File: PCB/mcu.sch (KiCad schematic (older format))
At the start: 50 parts, among them J1 DBG, P1 PC, P2 Link, P3 SSD1107, Q1 SSP6206, U1 USBLC6-2SC6, U2 USBLC6-2SC6, U3 STM32F103CBTx

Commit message: Update YAEMK
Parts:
- removed C39: 100n, prettylib:SMD-0603, symbol YAEMK:C
- removed D78: LED, prettylib:LED-0603, symbol YAEMK:LED
- added C3, C38: 100n, prettylib:SMD-0603, symbol YAEMK:C
- added D38, D39: DIODE, Diode_SMD:D_0603_1608Metric, symbol YAEMK:DIODE
- added Q2: Q_PNP_BCE, prettylib:SOT-23, symbol Device:Q_PNP_BCE
- added R14: 1k5, prettylib:SMD-0603, symbol YAEMK:R
- added R15, R16: 33, prettylib:SMD-0603, symbol YAEMK:R
- added R8: 120R, prettylib:SMD-0603, symbol YAEMK:R
- added S7: DFU, prettylib:SMD_Tacticle_Switch_TS24CA, symbol YAEMK:SW
- added U4: 24LC64, Package_SO:TSSOP-8_4.4x3mm_P0.65mm, symbol Memory_EEPROM:24LC64
- JP10, JP3, JP4, JP5, JP6, JP7, JP8, JP9: symbol YAEMK:SolderJumper_2_Open -> YAEMK-rescue:SolderJumper_2_Open-YAEMK
- Q1: symbol YAEMK:SSP6206 -> YAEMK-rescue:SSP6206-YAEMK
- R10: value 10k -> 1M
- R9: value 2k2 -> 1k5
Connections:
- net labels added: BOOT0_CHARGE
- net labels removed: MCU_LED
- wire segments 150 -> 181
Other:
- note added: "I2C EEPROM"
- note added: "Reset and DFU Bootloader Circuit"
- note removed: "Boot Mode"
- note removed: "Reset Button\n"
- moved on the sheet: C37, C42, C43, C44, C45, C46, C47, C48, C49, C56, C57, C59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

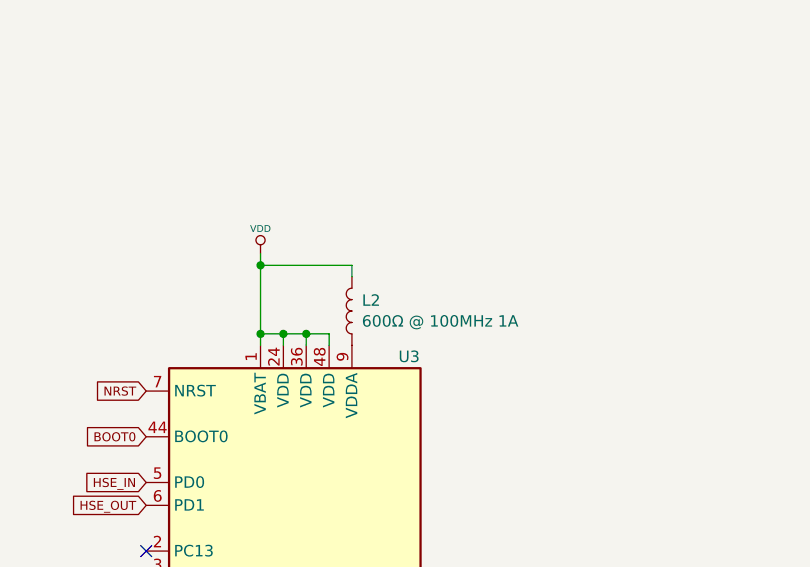
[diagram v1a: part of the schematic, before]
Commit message: Update YAEMK 1
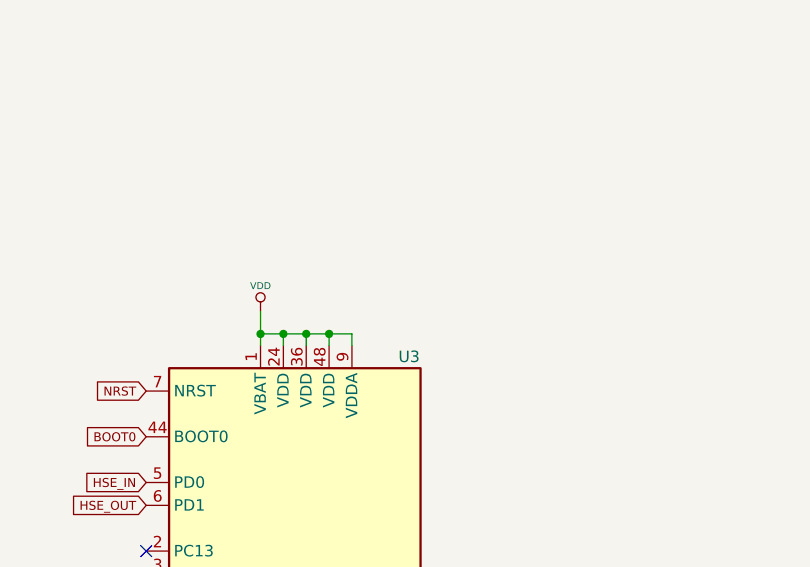
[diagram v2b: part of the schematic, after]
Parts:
- removed L2: 600Ω @ 100MHz 1A, prettylib:SMD-0603, symbol YAEMK:L
- HSE1: footprint prettylib:Crystal_SMD_EuroQuartz_MJ-4Pin_5.0x3.2mm -> Crystal:Crystal_SMD_3225-4Pin_3.2x2.5mm
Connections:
- net VDD: now also U3.9 (VDDA)
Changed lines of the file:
@@
 L YAEMK:VDD #PWR025
 U 1 1 5EA004DE
-P 8550 4450
-F 0 "#PWR025" H 8550 4550 30  0001 C CNN
-F 1 "VDD" H 8550 4560 30  0000 C CNN
-F 2 "" H 8550 4450 60  0000 C CNN
-F 3 "" H 8550 4450 60  0000 C CNN
-	1    8550 4450
+P 8550 4700
+F 0 "#PWR025" H 8550 4800 30  0001 C CNN
+F 1 "VDD" H 8550 4810 30  0000 C CNN
+F 2 "" H 8550 4700 60  0000 C CNN
+F 3 "" H 8550 4700 60  0000 C CNN
+	1    8550 4700
 	1    0    0    -1
 $EndComp
@@
 Wire Wire Line
 	8750 4800 8850 4800
-Wire Wire Line
-	8550 4450 8550 4500
 Wire Wire Line
 	8550 8000 8550 7900
@@
 F 0 "HSE1" H 14050 1300 50  0000 L CNN
 F 1 "8MHz" H 14050 1200 50  0000 L CNN
-F 2 "prettylib:Crystal_SMD_EuroQuartz_MJ-4Pin_5.0x3.2mm" H 14400 1050 50  0001 C CNN
+F 2 "Crystal:Crystal_SMD_3225-4Pin_3.2x2.5mm" H 14400 1050 50  0001 C CNN
 F 3 "~" H 14400 1050 50  0001 C CNN
 	1    14400 1050
@@
 	8650 4800 8750 4800
 $Comp
-L YAEMK:L L2
-U 1 1 5F849BB2
-P 8950 4700
-F 0 "L2" H 8907 4654 50  0000 R CNN
-F 1 "600Ω @ 100MHz 1A" H 8907 4745 50  0000 R CNN
-F 2 "prettylib:SMD-0603" H 8950 4700 50  0001 C CNN
-F 3 "~" H 8950 4700 50  0001 C CNN
-	1    8950 4700
-	-1   0    0    1
-$EndComp
-$Comp
 L YAEMK:VSS #PWR026
 U 1 1 5EAADE05
@@
 	1    0    0    -1
 $EndComp
-Wire Wire Line
-	8950 4550 8950 4500
-Wire Wire Line
-	8950 4500 8550 4500
-Connection ~ 8550 4500
-Wire Wire Line
-	8550 4500 8550 4800
 $Comp
 L YAEMK:USB_C_Receptacle_USB2.0 P1
@@
 Wire Wire Line
 	10350 7350 10150 7350
+Wire Wire Line
+	8550 4700 8550 4800
+Wire Wire Line
+	8950 4850 8950 4800
+Wire Wire Line
+	8950 4800 8850 4800
+Connection ~ 8850 4800
 $EndSCHEMATC

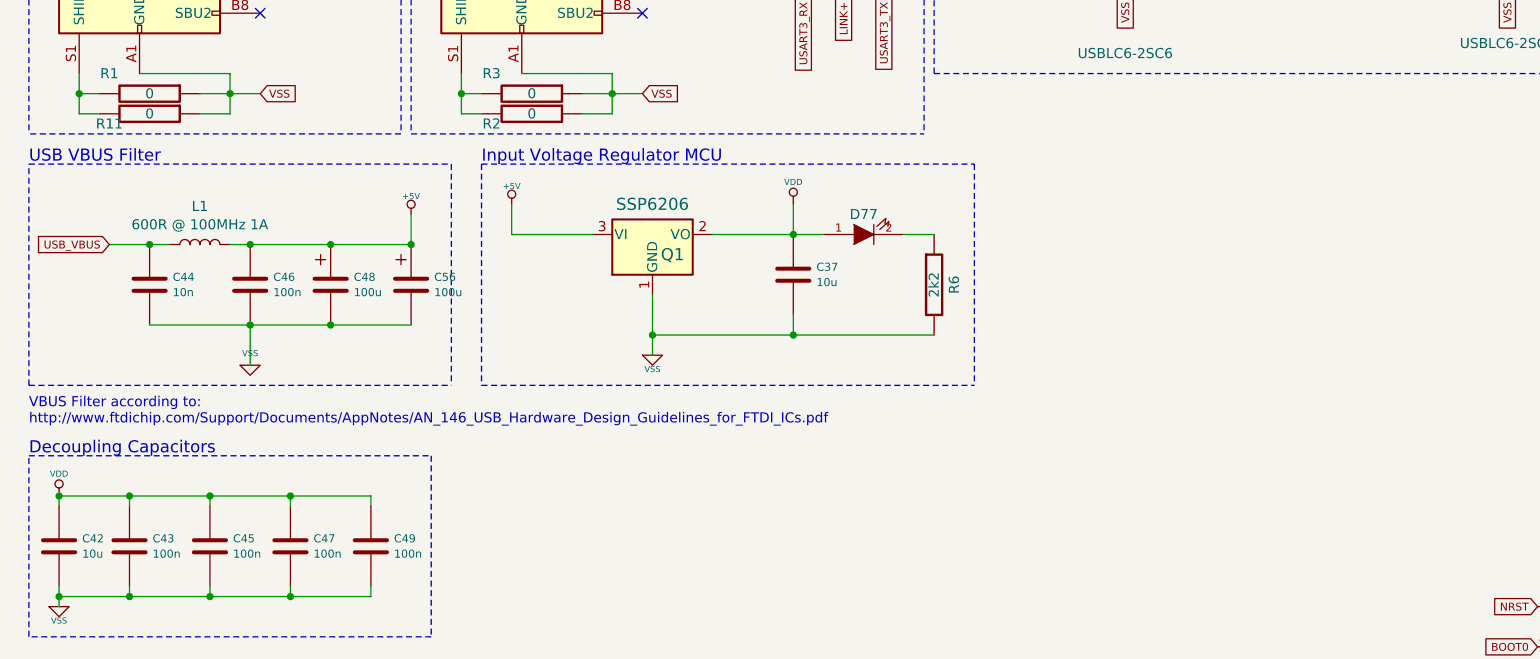
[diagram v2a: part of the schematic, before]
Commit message: Sync
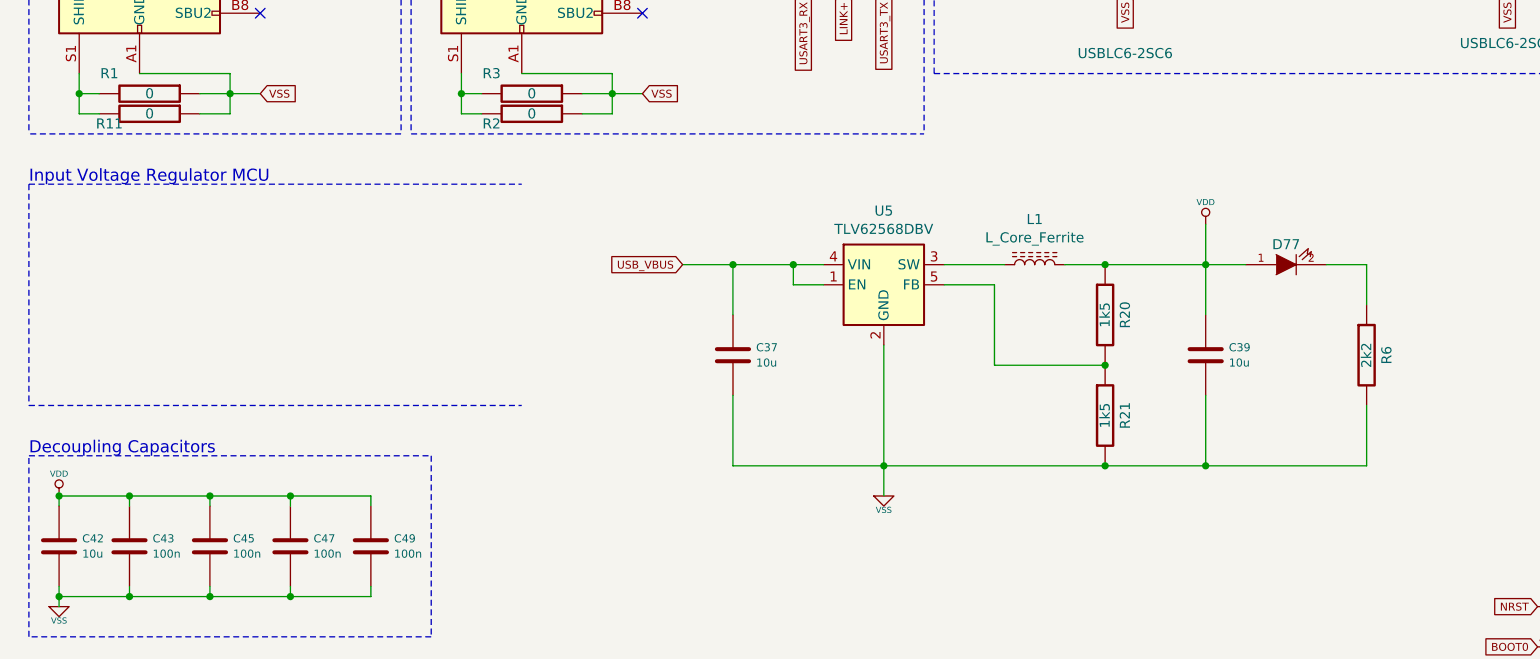
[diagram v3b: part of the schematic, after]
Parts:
- removed C44: 10n, prettylib:SMD-0603, symbol YAEMK:C
- removed C46: 100n, prettylib:SMD-0603, symbol YAEMK:C
- removed C48, C56: 100u, prettylib:CP_EIA-3528-12_Kemet-T_Pad1.50x2.35mm_HandSolder, symbol YAEMK:CT
- removed L1: 600R @ 100MHz 1A, prettylib:SMD-0603, symbol YAEMK:L
- removed Q1: SSP6206, prettylib:SOT-23, symbol YAEMK-rescue:SSP6206-YAEMK
- added C39: 10u, prettylib:SMD-0805, symbol YAEMK:C
- added L1: L_Core_Ferrite, Inductor_SMD:L_Taiyo-Yuden_MD-3030, symbol Device:L_Core_Ferrite
- added R20, R21: 1k5, prettylib:SMD-0603, symbol YAEMK:R
- added U5: TLV62568DBV, Package_TO_SOT_SMD:SOT-23-5, symbol Regulator_Switching:TLV62568DBV
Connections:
- net USB_VBUS: now also C37.1, U5.1 (EN), U5.4 (VIN)
- net VDD: now also C39.1, L1.2, R20.1; no longer C37.1
- net VSS: now also C39.2, R21.2, U5.2 (GND)
- new net: L1.1, U5.3 (SW)
- new net: R20.2, R21.1, U5.5 (FB)
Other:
- note removed: "USB VBUS Filter"
- note removed: "VBUS Filter according to:\nhttp://www.ftdichip.com/Support/Documents/AppNotes/AN_146_USB_Hardware_Design_Guidelines_for_FTDI_ICs.pdf"
- moved on the sheet: D77, R6
